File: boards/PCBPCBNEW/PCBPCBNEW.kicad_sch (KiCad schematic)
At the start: 71 parts, among them J1 Screw_Terminal_01x02, J4 Screw_Terminal_01x06, U1 SIC431AED-T1-GE3, U2 SIC431AED-T1-GE3, U3 SIC431AED-T1-GE3

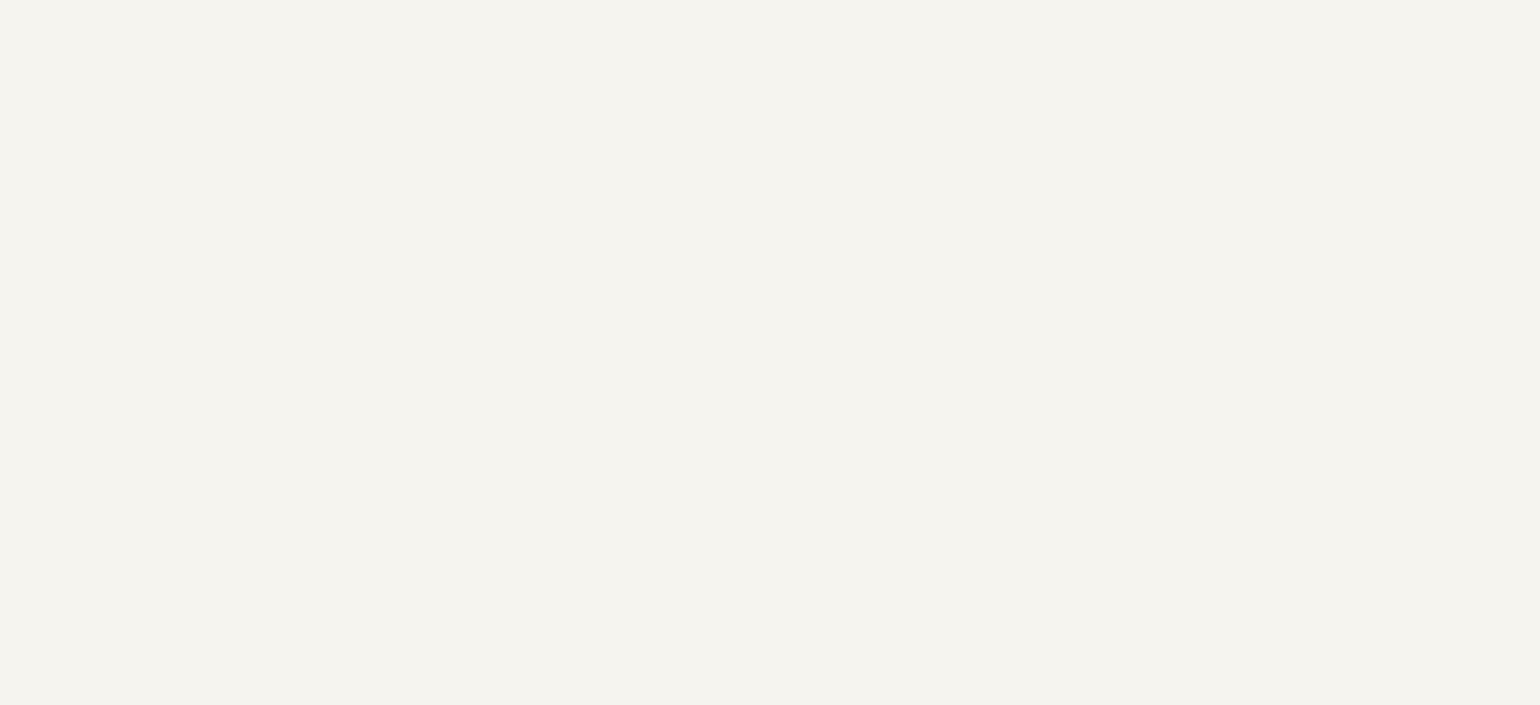
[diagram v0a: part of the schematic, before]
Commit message: pcbpcbnew2
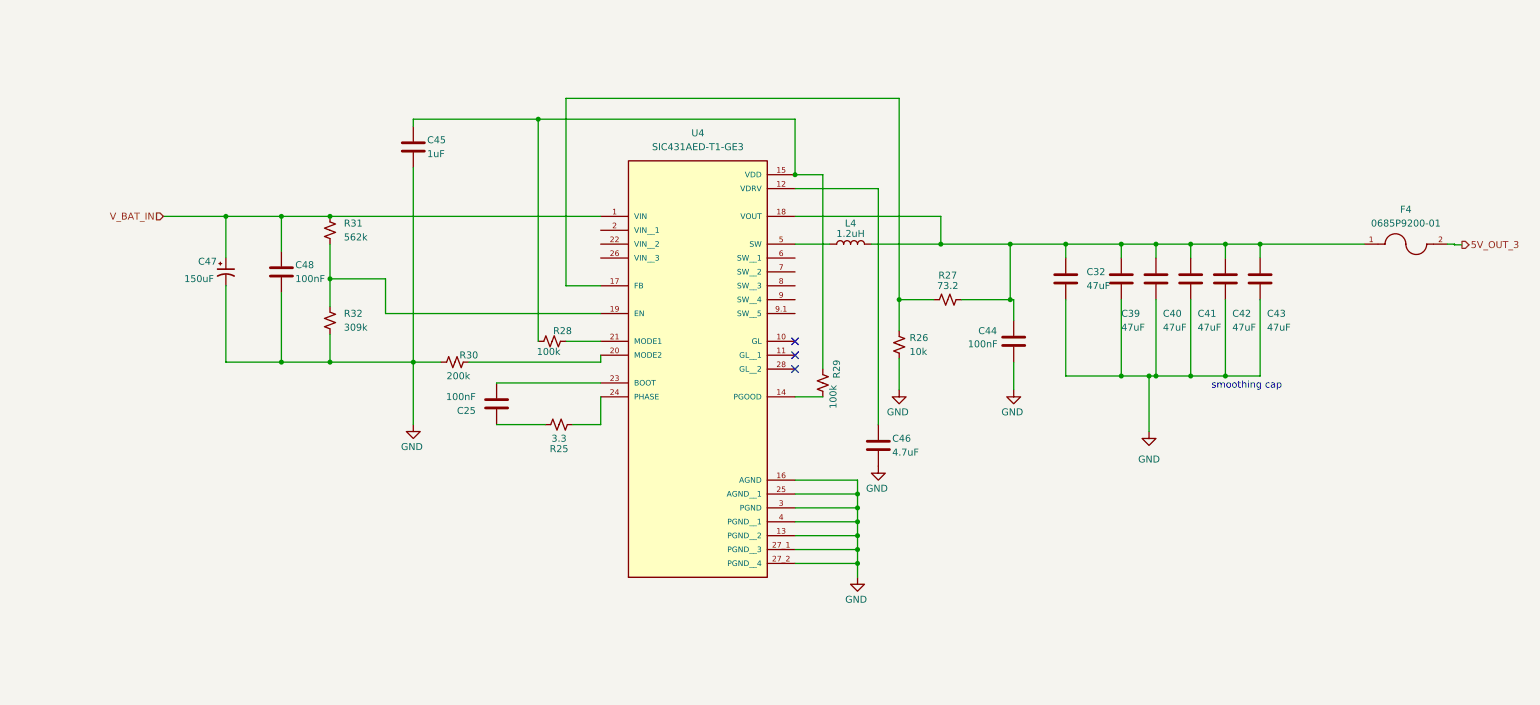
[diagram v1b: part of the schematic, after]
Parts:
- added C25, C44, C48: 100nF, Capacitor_SMD:C_0805_2012Metric, symbol Device:C
- added C32, C39, C40, C41, C42, C43: 47uF, Capacitor_SMD:C_0805_2012Metric, symbol Device:C
- added C45: 1uF, Capacitor_SMD:C_0805_2012Metric, symbol Device:C
- added C46: 4.7uF, Capacitor_SMD:C_0805_2012Metric, symbol Device:C
- added C47: 150uF, Capacitor_THT:CP_Radial_D12.5mm_P5.00mm, symbol Device:C_Polarized_Small_US
- added F4: 0685P9200-01, IRIS:FUSC3215X83N, symbol IRIS:0685P9200-01
- added L4: 1.2uH, Inductor_SMD:L_Vishay_IHLP-5050, symbol Device:L
- added R25: 3.3, Resistor_SMD:R_0805_2012Metric, symbol Device:R_Small_US
- added R26: 10k, Resistor_SMD:R_0805_2012Metric, symbol Device:R_Small_US
- added R27: 73.2, Resistor_SMD:R_0805_2012Metric, symbol Device:R_Small_US
- added R28, R29: 100k, Resistor_SMD:R_0805_2012Metric, symbol Device:R_Small_US
- added R30: 200k, Resistor_SMD:R_0805_2012Metric, symbol Device:R_Small_US
- added R31: 562k, Resistor_SMD:R_0805_2012Metric, symbol Device:R_Small_US
- added R32: 309k, Resistor_SMD:R_0805_2012Metric, symbol Device:R_Small_US
- added U4: SIC431AED-T1-GE3, SIC431AED_T1_GE3:REGULATOR_SIC431AED-T1-GE3, symbol SIC431AED-T1-GE3:SIC431AED-T1-GE3
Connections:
- net 5V_OUT_3: now also F4.2
- net GND: now also C32.2, C39.2, C40.2, C41.2, C42.2, C43.2, C44.2, C45.2, C46.2, C47.2, C48.2, R26.2, R30.1, R32.2, U4.13 (PGND__2), U4.16 (AGND), U4.25 (AGND__1), U4.27_1 (PGND__3), U4.27_2 (PGND__4), U4.3 (PGND), U4.4 (PGND__1)
- net V_BAT_IN: now also C47.1, C48.1, R31.1, U4.1 (VIN)
- new net: C32.1, C39.1, C40.1, C41.1, C42.1, C43.1, C44.1, F4.1, L4.2, R27.2, U4.18 (VOUT)
- new net: C46.1, U4.12 (VDRV)
- new net: R26.1, R27.1, U4.17 (FB)
- new net: R31.2, R32.1, U4.19 (EN)
- new net: C45.1, R28.1, R29.1, U4.15 (VDD)
- new net: C25.1, R25.2
- new net: C25.2, U4.23 (BOOT)
- new net: L4.1, U4.5 (SW)
- new net: R29.2, U4.14 (PGOOD)
- new net: R25.1, U4.24 (PHASE)
- new net: R30.2, U4.20 (MODE2)
- new net: R28.2, U4.21 (MODE1)
- no-connect marks 3 -> 6
